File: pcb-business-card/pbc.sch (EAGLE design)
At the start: 25 parts, among them IC1 NET2272REV1A-BCF, J1 CON2, U1 MEGA32U4-MU, U2 RT9193-33GB, U5 TMP117AIYBGR

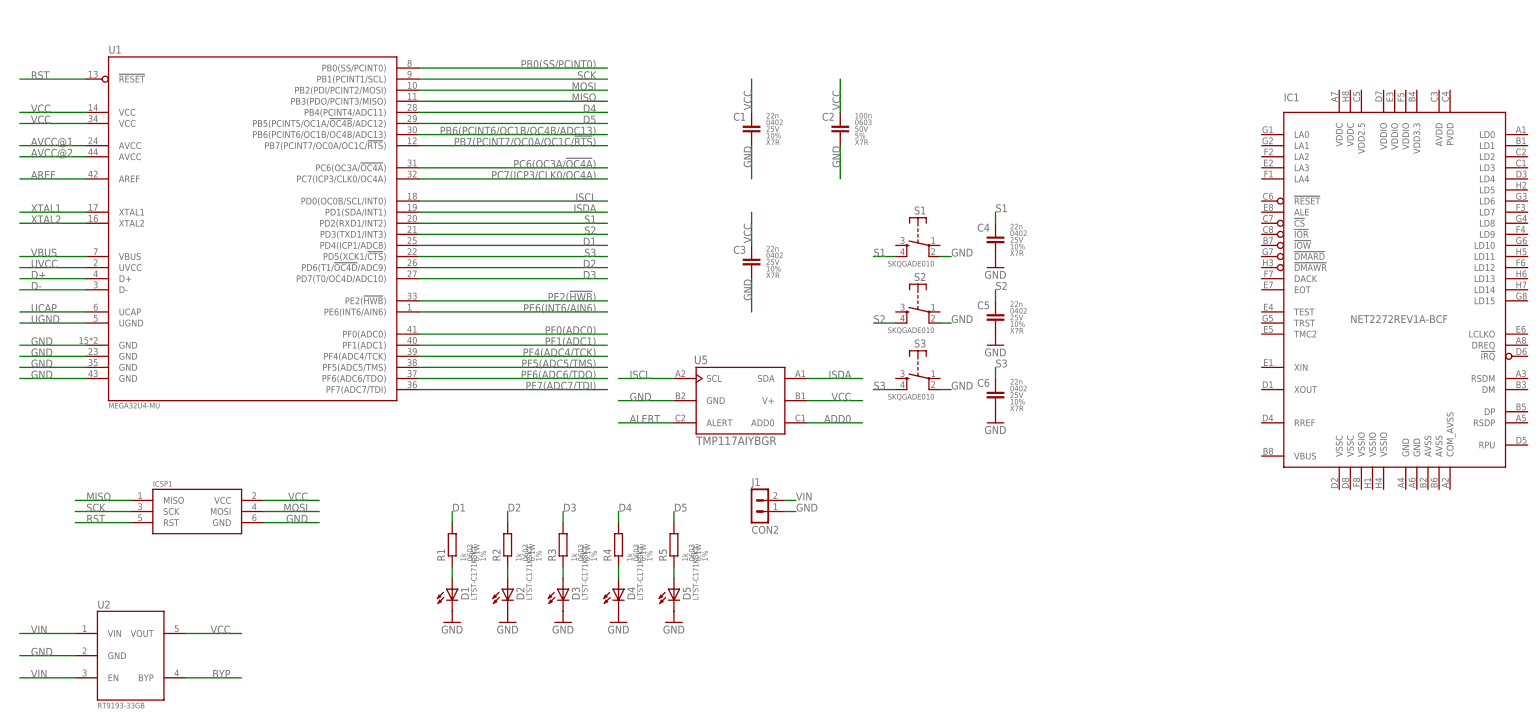
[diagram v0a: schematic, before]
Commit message: Created gerbers
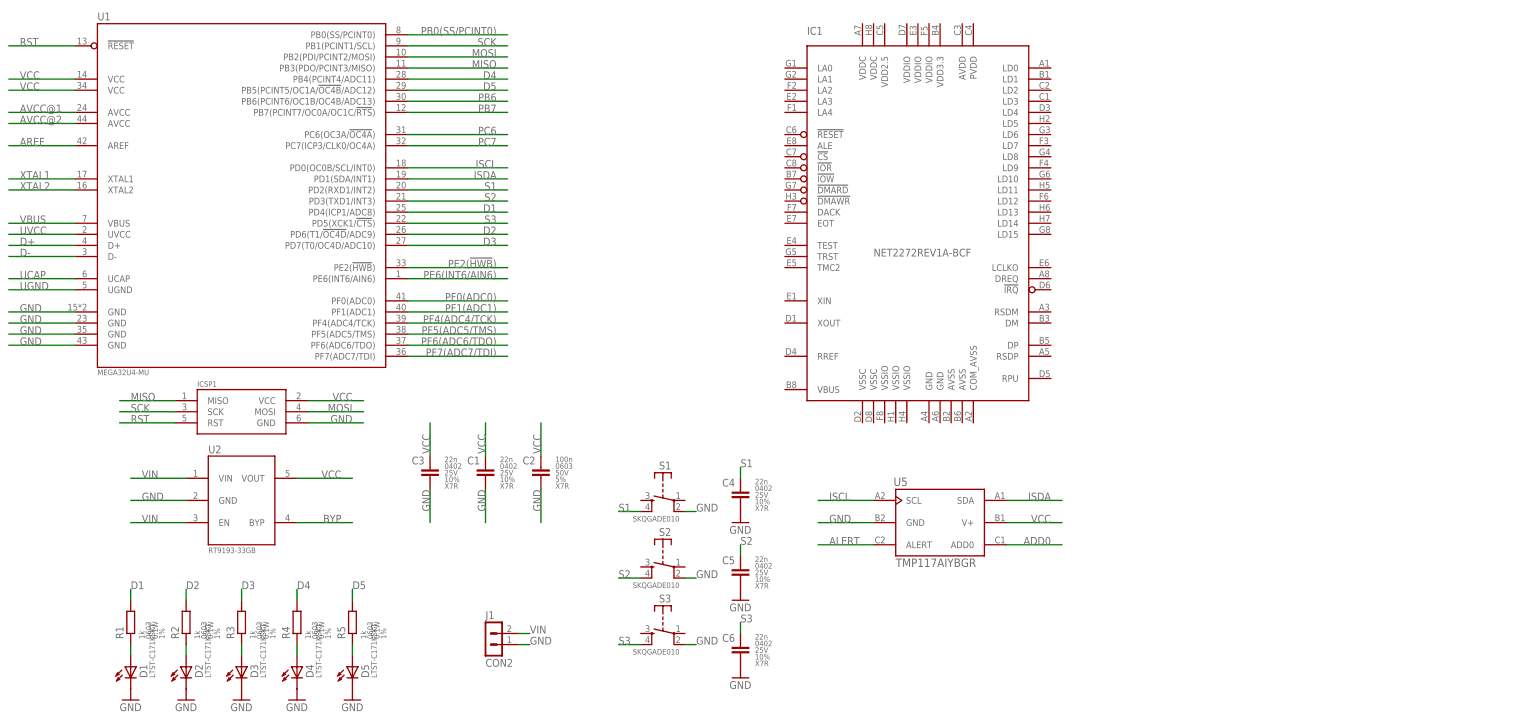
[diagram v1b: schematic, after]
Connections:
- net PB6(PCINT6/OC1B/OC4B/ADC13) renamed PB6
- net PB7(PCINT7/OC0A/OC1C/!RTS!) renamed PB7
- net PC6(OC3A/!OC4A!) renamed PC6
- net PC7(ICP3/CLK0/OC4A) renamed PC7
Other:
- moved on the sheet: C1, C2, C3, C4, C5, C6, D1, D2, D3, D4, D5, IC1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
